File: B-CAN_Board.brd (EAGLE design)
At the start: 40.3 x 59.7 mm, 3 parts, among them X1 GLX-S-88M

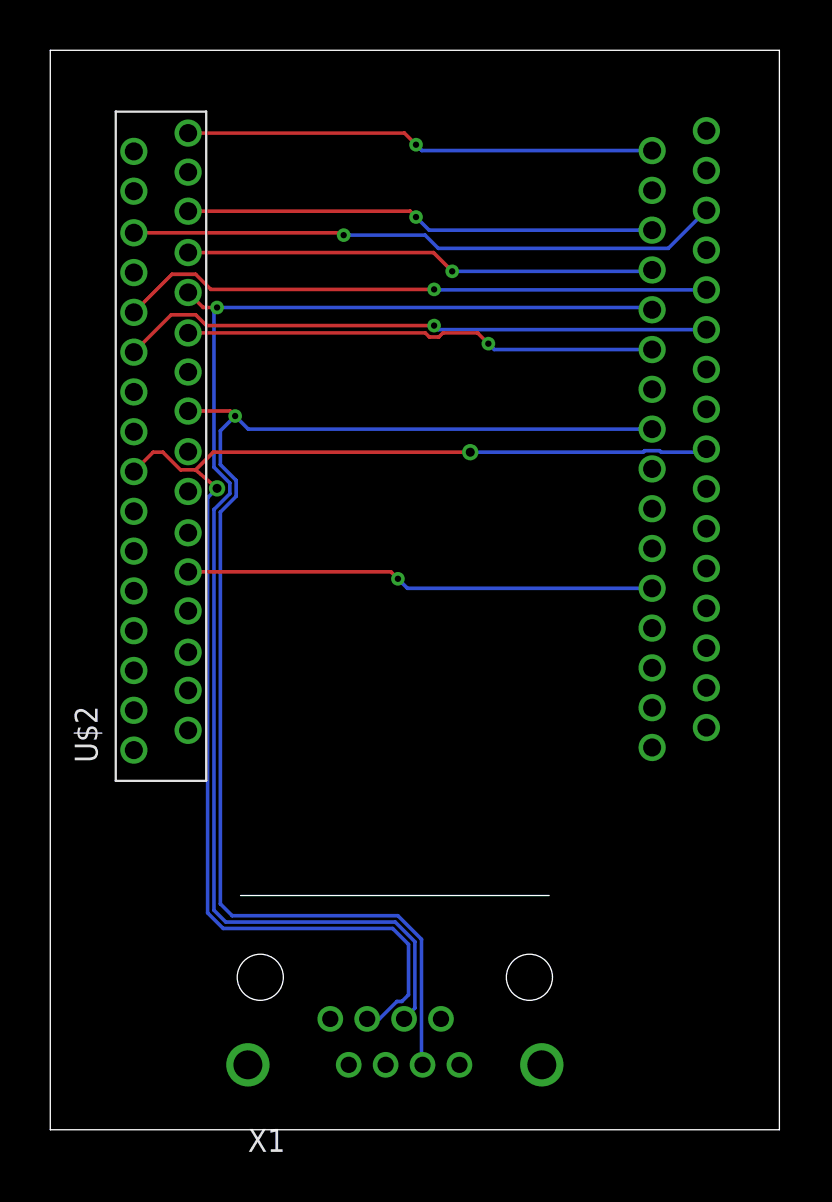
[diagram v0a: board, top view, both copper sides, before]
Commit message: God this used to look so ugly, lets make it nice
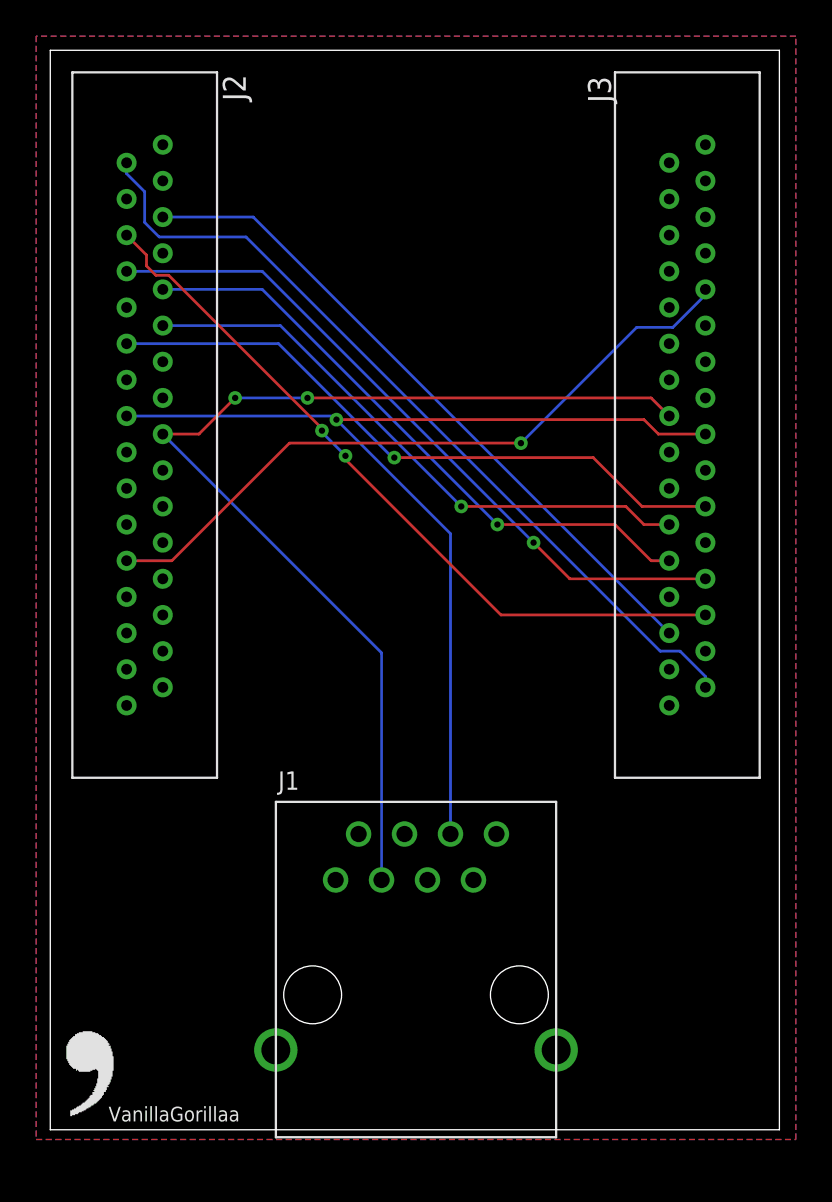
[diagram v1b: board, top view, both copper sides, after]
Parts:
- removed U$1: 670-2297-ND, 670-2297-ND:670-2297-ND
- removed X1: GLX-S-88M, con-kycon:GLX-S-88M
- added J1: RA-RJ45RA, comma.ai:RA-RJ45
- added J2, J3: MX34032UF2, MX34032UF2:MX34032UF2
- U$2: value 670-2910-ND -> (none); device 670-2910-ND:670-2910-ND -> comma.ai:LOGO
- moved U$2 35.6 mm to (18.0, 3.00), turned to 0 degrees
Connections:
- removed net N$1: U$1.P$14, U$2.P$14
- removed net N$10: U$1.P$29, U$2.P$29
- removed net N$11: U$1.P$30, U$2.P$30
- removed net N$2: U$1.P$8, U$2.P$8, X1.3
- removed net N$3: U$1.P$11, U$2.P$11
- removed net N$4: U$1.P$12, U$2.P$12
- removed net N$5: U$1.P$32, U$2.P$32
- removed net N$6: U$1.P$21, U$2.P$21
- removed net N$7: U$1.P$25, U$2.P$25, X1.6
- removed net N$8: U$1.P$27, U$2.P$27
- removed net N$9: U$1.P$28, U$2.P$28, X1.5
- new net B-CAN_H: J1.6, J2.P25, J3.P25
- new net B-CAN_L: J1.3, J2.P8, J3.P8
- new net BUS-DATA: J2.P29, J3.P29
- new net GND: J2.P28, J3.P28
- new net IG2_A/C: J2.P32, J3.P32
- new net RR_DEF_RLY_CL-: J2.P21, J3.P21
- new net SENSOR_COM: J2.P12, J3.P12
- new net SOL_IN: J2.P14, J3.P14
- new net SOL_OUT: J2.P30, J3.P30
- new net TAM: J2.P11, J3.P11
- new net TR: J2.P27, J3.P27
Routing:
- net N$9: track 76.5 -> 0.00 mm, vias 1 -> 0
- net N$2: track 76.0 -> 0.00 mm, vias 2 -> 0
- net N$7: track 73.0 -> 0.00 mm, vias 1 -> 0
- net B-CAN_L: track 0.00 -> 58.9 mm, vias 0 -> 2
- net B-CAN_H: track 0.00 -> 57.9 mm, vias 0 -> 1
- net IG2_A/C: track 0.00 -> 45.7 mm
- net SOL_OUT: track 0.00 -> 41.3 mm, vias 0 -> 2
- net BUS-DATA: track 0.00 -> 39.0 mm, vias 0 -> 1
- net RR_DEF_RLY_CL-: track 0.00 -> 38.4 mm, vias 0 -> 1
- net SOL_IN: track 0.00 -> 37.5 mm
- net TR: track 0.00 -> 35.7 mm, vias 0 -> 1
- net SENSOR_COM: track 0.00 -> 34.2 mm, vias 0 -> 1
- net N$4: track 32.9 -> 0.00 mm, vias 1 -> 0
- net N$1: track 32.9 -> 0.00 mm, vias 1 -> 0
- net N$3: track 32.9 -> 0.00 mm, vias 1 -> 0
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- added copper zone on layer 1, net GND
- added copper zone on layer 16, net GND
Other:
- board text added: "VanillaGorillaa"
